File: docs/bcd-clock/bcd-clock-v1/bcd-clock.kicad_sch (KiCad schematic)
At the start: 41 parts, among them P1 (UART on the board), P2 (NMEA / NTP device), Q1 8550, Q2 8550, Q3 8550, Q4 8550, Q7 8550, U1 DS1302, U2 STC15W408AS, Y1 32768

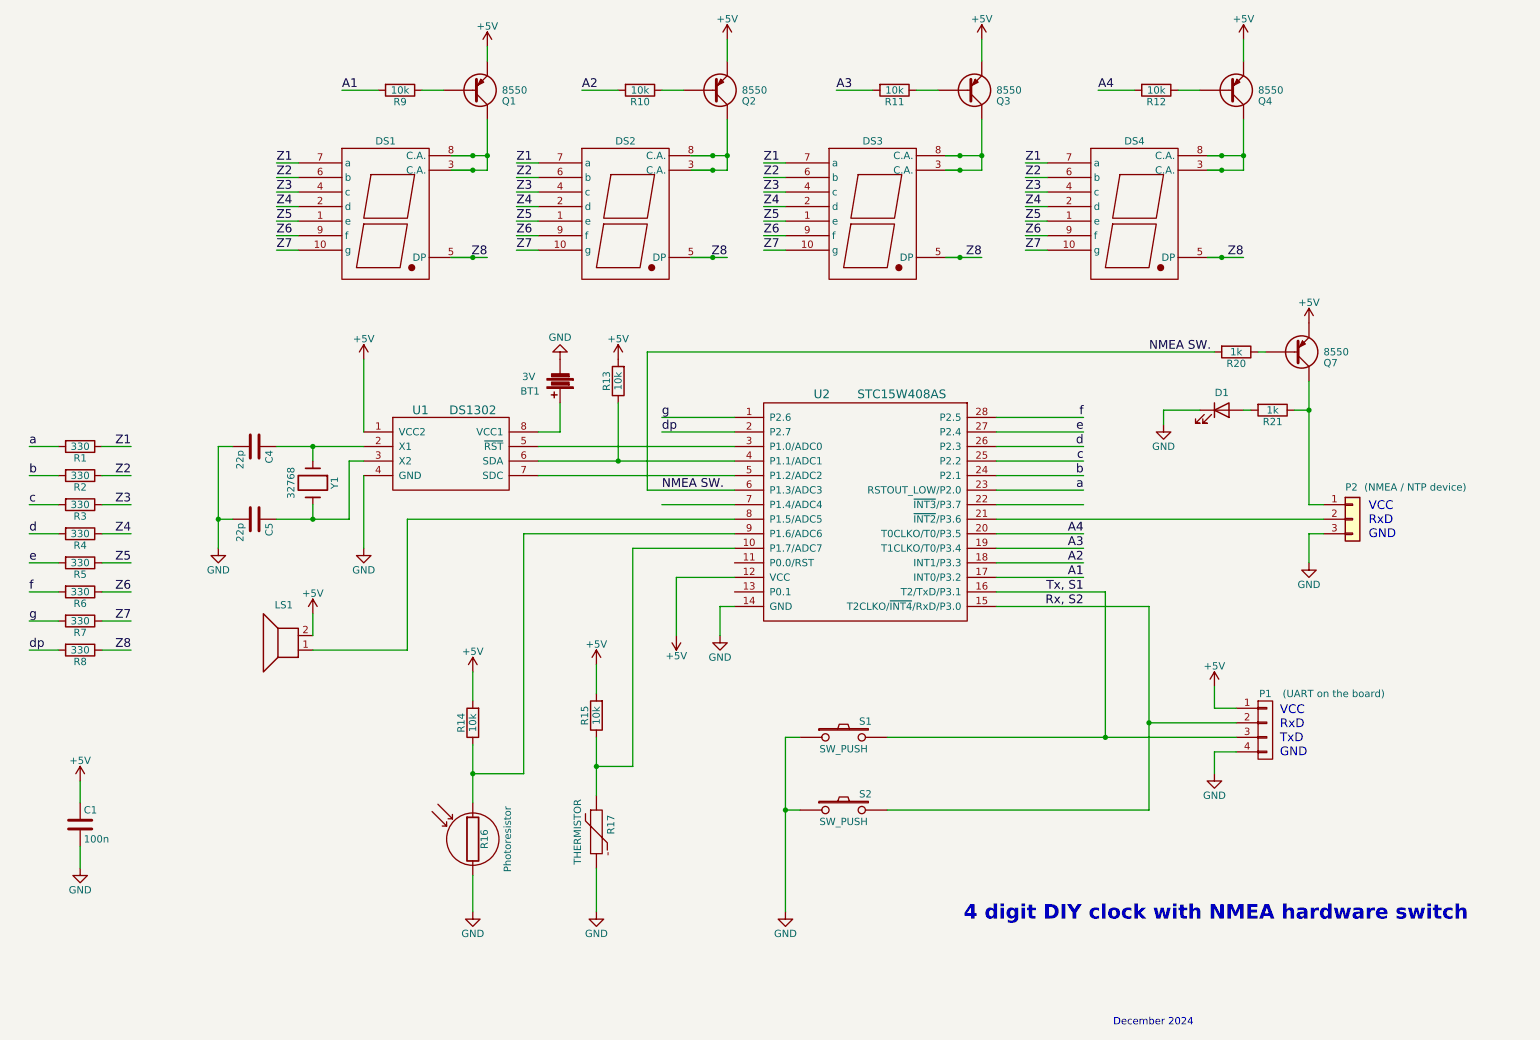
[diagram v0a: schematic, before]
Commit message: Updated documentation
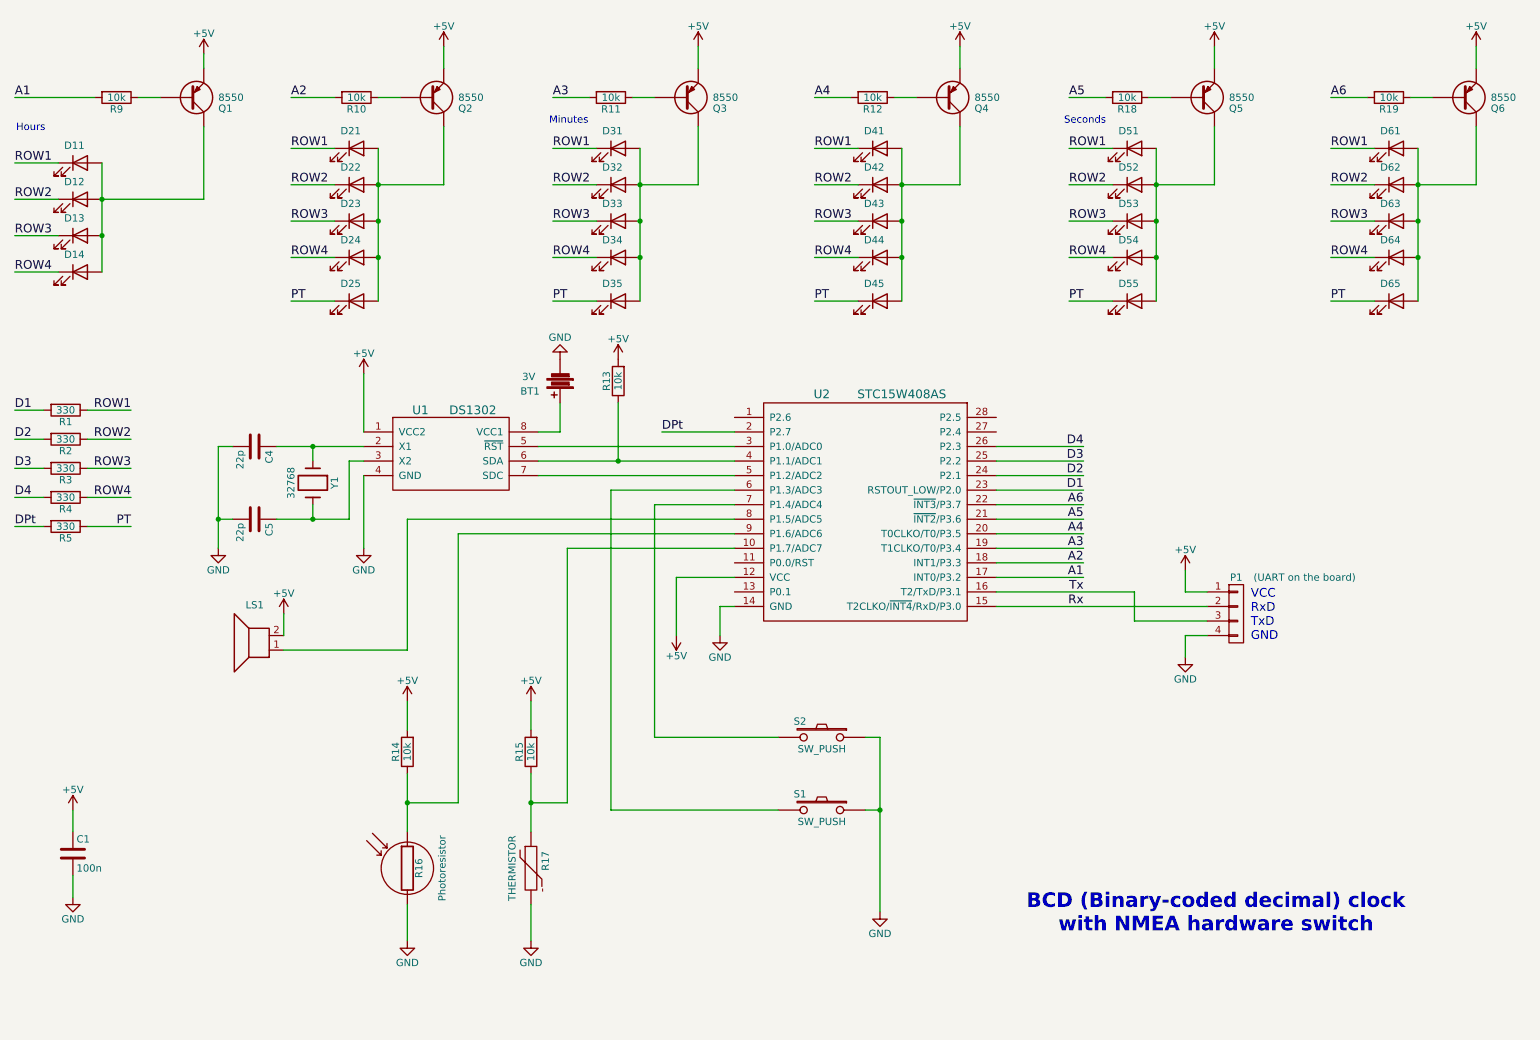
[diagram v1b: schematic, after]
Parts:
- removed D1: LED, symbol Device:LED
- removed DS1, DS2, DS3, DS4: 7SEGMENTS, symbol stc_diyclock-rescue:7SEGMENTS
- removed P2: (NMEA / NTP device), symbol Connector_Generic:Conn_01x03
- removed Q7: 8550, TO-92, symbol stc_diyclock-rescue:S8550
- removed R20, R21: 1k, symbol stc_diyclock-rescue:R
- removed R6, R7, R8: 330, symbol stc_diyclock-rescue:R
- added D11, D12, D13, D14, D21, D22, D23, D24, D25, D31, D32, D33, D34, D35, D41, D42, D43, D44, D45, D51, D52, D53, D54, D55, D61, D62, D63, D64, D65: LED, LED_THT:LED_D3.0mm, symbol Device:LED
- added Q5, Q6: 8550, TO-92, symbol stc_diyclock-rescue:S8550
- added R18: 10k, symbol stc_diyclock-rescue:R
- added R19: 10k, Resistor_THT:R_Axial_DIN0204_L3.6mm_D1.6mm_P1.90mm_Vertical, symbol stc_diyclock-rescue:R
- P1: footprint (none) -> Connector_PinHeader_2.54mm:PinHeader_1x04_P2.54mm_Vertical
- R1, R10, R11, R12, R13, R14, R15, R2, R3, R4, R5, R9: footprint (none) -> Resistor_THT:R_Axial_DIN0204_L3.6mm_D1.6mm_P1.90mm_Vertical
- renumbered S2 to S1, S1 to S2
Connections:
- net   : no longer U2.7 (P1.4/ADC4)
- net +5V: now also Q5.1 (E), Q6.1 (E)
- net at Q3.3 (C): now also D31.2 (A), D32.2 (A), D33.2 (A), D34.2 (A), D35.2 (A)
- net at Q4.3 (C): now also D41.2 (A), D42.2 (A), D43.2 (A), D44.2 (A), D45.2 (A)
- net at Q2.3 (C): now also D21.2 (A), D22.2 (A), D23.2 (A), D24.2 (A), D25.2 (A)
- net A5: now reaches U2.21 (~{INT2}/P3.6)
- net A5: now also R18.2
- net A6: now reaches U2.22 (~{INT3}/P3.7)
- net A6: now also R19.2
- net at Q1.3 (C): now also D11.2 (A), D12.2 (A), D13.2 (A), D14.2 (A)
- net NMEA SW.: no longer names the net of U2.6 (P1.3/ADC3)
- net NMEA SW.: now also S1.2
- net Rx, S2 renamed Rx
- net Rx: no longer S1.2
- net Tx, S1 renamed Tx
- net Tx: no longer S2.2
- net Z1 renamed ROW1
- net ROW1: now also D11.1 (K), D21.1 (K), D31.1 (K), D41.1 (K), D51.1 (K), D61.1 (K)
- net Z2 renamed ROW2
- net ROW2: now also D12.1 (K), D22.1 (K), D32.1 (K), D42.1 (K), D52.1 (K), D62.1 (K)
- net Z3 renamed ROW3
- net ROW3: now also D13.1 (K), D23.1 (K), D33.1 (K), D43.1 (K), D53.1 (K), D63.1 (K)
- net Z4 renamed ROW4
- net ROW4: now also D14.1 (K), D24.1 (K), D34.1 (K), D44.1 (K), D54.1 (K), D64.1 (K)
- net Z5 renamed PT
- net PT: now also D25.1 (K), D35.1 (K), D45.1 (K), D55.1 (K), D65.1 (K)
- net a renamed D1
- net b renamed D2
- net c renamed D3
- net d renamed D4
- net dp renamed DPt
- net DPt: now also R5.2
- net e: no longer names the net of U2.27 (P2.4)
- net e: no longer R5.2
- net f: no longer names the net of U2.28 (P2.5)
- net g: no longer names the net of U2.1 (P2.6)
- new net: D61.2 (A), D62.2 (A), D63.2 (A), D64.2 (A), D65.2 (A), Q6.3 (C)
- new net: D51.2 (A), D52.2 (A), D53.2 (A), D54.2 (A), D55.2 (A), Q5.3 (C)
- new net: S2.2, U2.7 (P1.4/ADC4)
- new net: Q6.2 (B), R19.1
- new net: Q5.2 (B), R18.1
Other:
- note added: "BCD (Binary-coded decimal) clock with NMEA hardware switch"
- note added: "Hours"
- note added: "Minutes"
- note added: "Seconds"
- note removed: "4 digit DIY clock with NMEA hardware switch"
- note removed: "December 2024"
- note removed: "VCC RxD GND"
- company: (none) -> Yuri
- moved on the sheet: C1, LS1, P1, Q1, Q2, Q3, Q4, R1, R10, R11, R12, R14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
